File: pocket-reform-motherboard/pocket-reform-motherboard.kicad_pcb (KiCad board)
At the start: 2 copper layers, 130 x 80 mm, 20 parts, among them J1 PWR, J2 Micro_SD_Card_Det, J3 USB_C_Receptacle, J4 AudioJack4, J5 USB_C_Receptacle, J6 USBINT, J7 HDMI_D_1.4, J8 SIM, U1 reform2-som-connector, U2 MPCIE-Socket-reform-motherboa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, U3 TUSB4041I, U4 WM8960, U6 MPCIE-Socket-reform-motherboa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

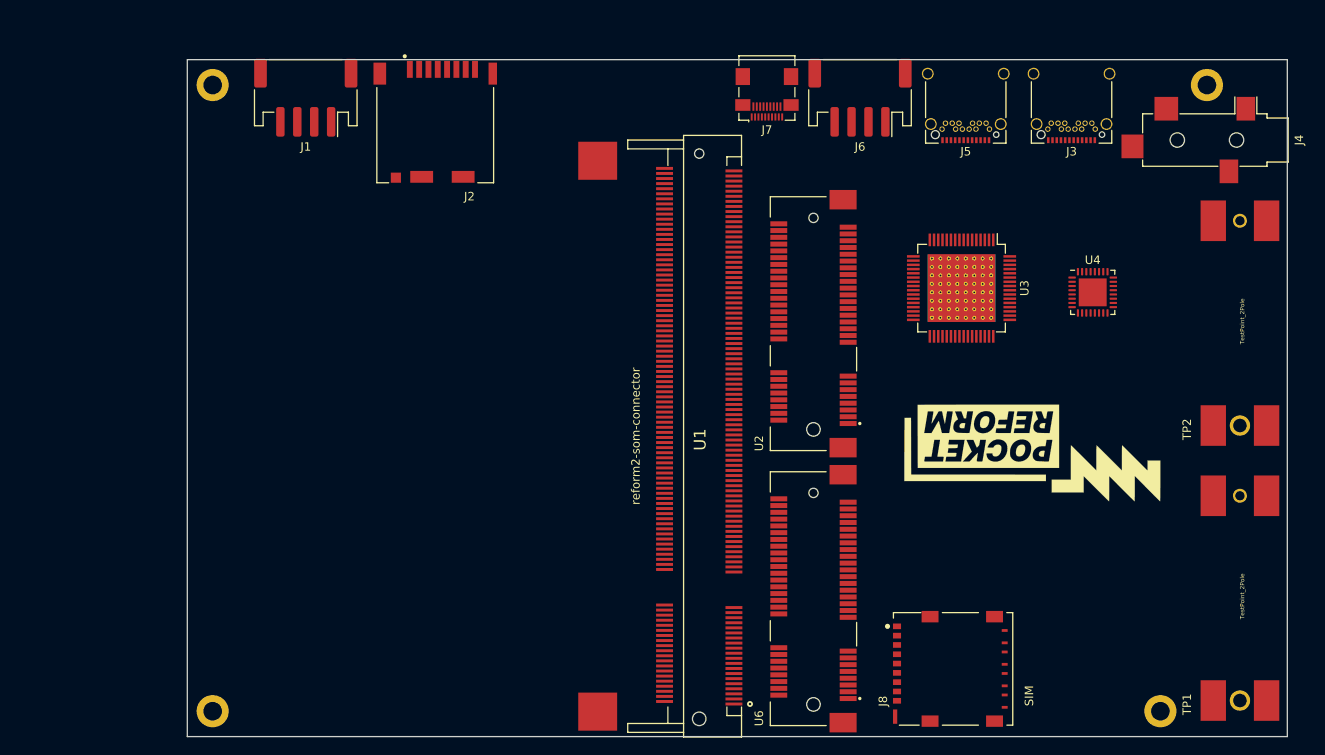
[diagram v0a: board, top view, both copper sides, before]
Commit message: motherboard D-1 first schematic and placement
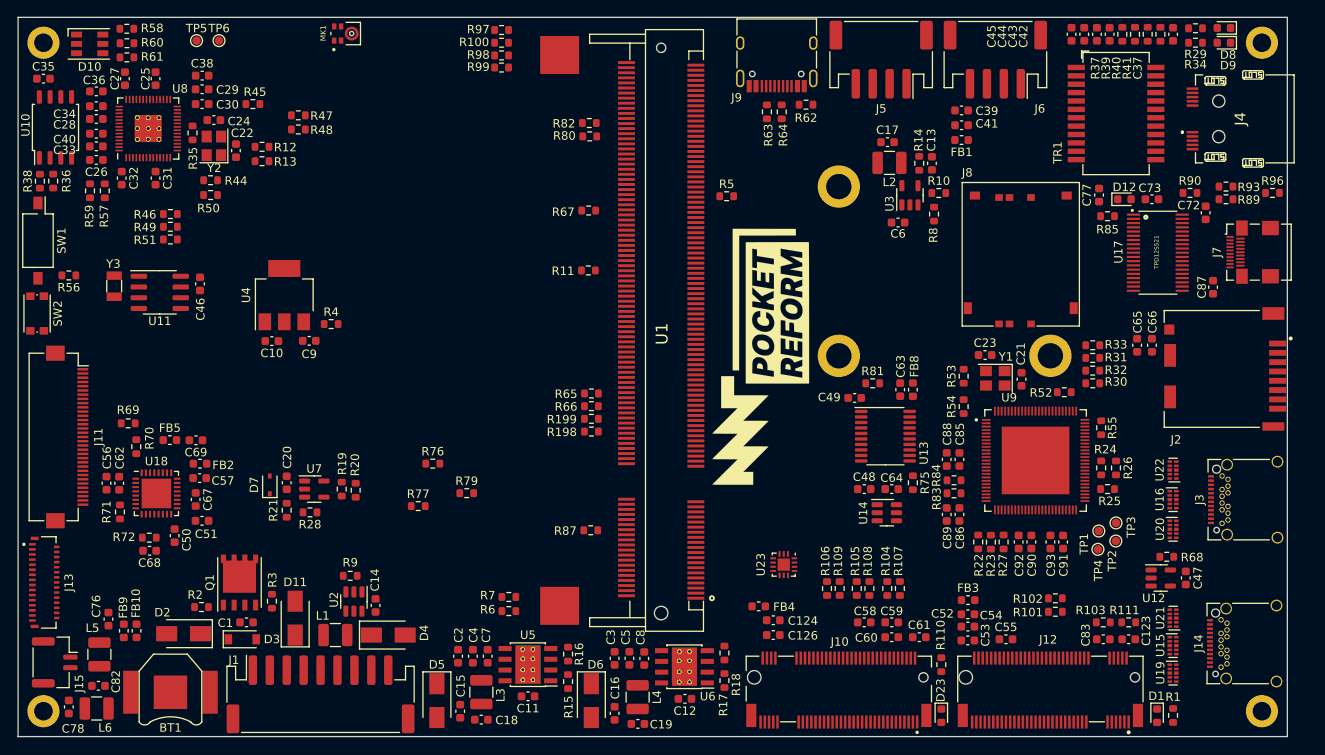
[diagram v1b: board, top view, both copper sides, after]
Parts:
- added BT1: V364, Battery:BatteryHolder_Keystone_2998_1x6.8mm, F.Cu at (77.0, 146.8)
- added C1: 0.1uF, Capacitor_SMD:C_0603_1608Metric, F.Cu at (86.0, 138.5)
- added C10: 1uF, Capacitor_SMD:C_0603_1608Metric, F.Cu at (89.0, 105.3)
- added C11: 10nF, Capacitor_SMD:C_0603_1608Metric, F.Cu at (119.3, 147.2)
- added C12: 10nF, Capacitor_SMD:C_0603_1608Metric, F.Cu at (137.8, 147.5)
- added C123: 47uF, Capacitor_SMD:C_0603_1608Metric, F.Cu at (190.2, 140.5)
- added C124: 47uF, Capacitor_SMD:C_0603_1608Metric, F.Cu at (148.2, 138.2)
- added C126: 47uF, Capacitor_SMD:C_0603_1608Metric, F.Cu at (148.2, 140.0)
- added C13: 12pF, Capacitor_SMD:C_0603_1608Metric, F.Cu at (167.0, 84.2)
- added C14: 68uF, Capacitor_SMD:C_0603_1608Metric, F.Cu at (101.2, 136.5)
- added C15: 330uF, Capacitor_SMD:C_0603_1608Metric, F.Cu at (111.2, 149.0)
- added C16: 330uF, Capacitor_SMD:C_0603_1608Metric, F.Cu at (129.5, 149.2)
- added C17: 10uF, Capacitor_SMD:C_0603_1608Metric, F.Cu at (161.8, 81.8)
- added C18: 10nF, Capacitor_SMD:C_0603_1608Metric, F.Cu at (113.8, 150.0)
- added C19: 10nF, Capacitor_SMD:C_0603_1608Metric, F.Cu at (132.2, 150.5)
- added C2: 4.7uF, Capacitor_SMD:C_0603_1608Metric, F.Cu at (111.0, 142.5)
- added C20: 1uF, Capacitor_SMD:C_0603_1608Metric, F.Cu at (90.8, 122.0)
- added C21: 18pF, Capacitor_SMD:C_0603_1608Metric, F.Cu at (177.6, 109.8)
- added C22: 27pF, Capacitor_SMD:C_0603_1608Metric, F.Cu at (84.8, 82.8)
- added C23: 18pF, Capacitor_SMD:C_0603_1608Metric, F.Cu at (173.3, 106.9)
- added C24: 27pF, Capacitor_SMD:C_0603_1608Metric, F.Cu at (82.1, 79.1)
- added C25: 0.1uF, Capacitor_SMD:C_0603_1608Metric, F.Cu at (75.2, 74.2)
- added C26: 1uF, Capacitor_SMD:C_0603_1608Metric, F.Cu at (68.2, 83.8)
- added C27: 0.1uF, Capacitor_SMD:C_0603_1608Metric, F.Cu at (71.6, 74.2)
- added C28: 0.1uF, Capacitor_SMD:C_0603_1608Metric, F.Cu at (68.2, 79.0)
- added C29: 0.1uF, Capacitor_SMD:C_0603_1608Metric, F.Cu at (80.8, 75.5)
- added C3: 4.7uF, Capacitor_SMD:C_0603_1608Metric, F.Cu at (129.5, 142.8)
- added C30: 0.1uF, Capacitor_SMD:C_0603_1608Metric, F.Cu at (80.8, 77.2)
- added C31: 0.1uF, Capacitor_SMD:C_0603_1608Metric, F.Cu at (75.2, 86.0)
- added C32: 0.1uF, Capacitor_SMD:C_0603_1608Metric, F.Cu at (71.2, 86.0)
- added C33: 0.1uF, Capacitor_SMD:C_0603_1608Metric, F.Cu at (68.2, 82.2)
- added C34: 1uF, Capacitor_SMD:C_0603_1608Metric, F.Cu at (68.2, 77.5)
- added C35: 0.1uF, Capacitor_SMD:C_0603_1608Metric, F.Cu at (62.0, 74.2)
- added C36: 1uF, Capacitor_SMD:C_0603_1608Metric, F.Cu at (68.2, 75.8)
- added C37: 1nF, Capacitor_SMD:C_0603_1608Metric, F.Cu at (195.5, 69.0)
- added C38: 0.1uF, Capacitor_SMD:C_0603_1608Metric, F.Cu at (80.8, 73.9)
- added C39: 10uF, Capacitor_SMD:C_0603_1608Metric, F.Cu at (170.5, 78.0)
- added C4: 4.7uF, Capacitor_SMD:C_0603_1608Metric, F.Cu at (112.8, 142.5)
- added C40: 0.1uF, Capacitor_SMD:C_0603_1608Metric, F.Cu at (68.2, 80.8)
- added C41: 0.1uF, Capacitor_SMD:C_0603_1608Metric, F.Cu at (170.5, 79.8)
- added C42: 0.1uF, Capacitor_SMD:C_0603_1608Metric, F.Cu at (188.0, 69.0)
- added C43: 0.1uF, Capacitor_SMD:C_0603_1608Metric, F.Cu at (186.5, 69.0)
- added C44: 0.1uF, Capacitor_SMD:C_0603_1608Metric, F.Cu at (185.0, 69.0)
- added C45: 0.1uF, Capacitor_SMD:C_0603_1608Metric, F.Cu at (183.5, 69.0)
- added C46: 0.1uF, Capacitor_SMD:C_0603_1608Metric, F.Cu at (80.5, 98.5)
- added C47: 0.1uF, Capacitor_SMD:C_0603_1608Metric, F.Cu at (197.0, 133.2)
- added C48: 0.1uF, Capacitor_SMD:C_0603_1608Metric, F.Cu at (159.0, 122.8)
- added C49: 0.1uF, Capacitor_SMD:C_0603_1608Metric, F.Cu at (157.9, 112.0)
- added C5: 4.7uF, Capacitor_SMD:C_0603_1608Metric, F.Cu at (131.2, 142.8)
- added C50: 0.1uF, Capacitor_SMD:C_0603_1608Metric, F.Cu at (77.5, 128.2)
- added C51: 10uF, Capacitor_SMD:C_0603_1608Metric, F.Cu at (80.7, 126.5)
- added C52: 10nF, Capacitor_SMD:C_0603_1608Metric, F.Cu at (171.2, 137.6)
- added C53: 0.1uF, Capacitor_SMD:C_0603_1608Metric, F.Cu at (171.2, 140.6)
- added C54: 0.1uF, Capacitor_SMD:C_0603_1608Metric, F.Cu at (171.2, 139.0)
- added C55: 0.1uF, Capacitor_SMD:C_0603_1608Metric, F.Cu at (175.8, 140.5)
- added C56: 10uF, Capacitor_SMD:C_0603_1608Metric, F.Cu at (69.5, 122.0)
- added C57: 0.1uF, Capacitor_SMD:C_0603_1608Metric, F.Cu at (80.5, 121.5)
- added C58: 10nF, Capacitor_SMD:C_0603_1608Metric, F.Cu at (159.0, 138.5)
- added C59: 0.1uF, Capacitor_SMD:C_0603_1608Metric, F.Cu at (162.2, 138.5)
- added C6: 4.7uF, Capacitor_SMD:C_0603_1608Metric, F.Cu at (163.0, 91.2)
- added C60: 0.1uF, Capacitor_SMD:C_0603_1608Metric, F.Cu at (162.2, 140.2)
- added C61: 0.1uF, Capacitor_SMD:C_0603_1608Metric, F.Cu at (165.5, 140.2)
- added C62: 0.1uF, Capacitor_SMD:C_0603_1608Metric, F.Cu at (71.0, 122.1)
- added C63: 0.1uF, Capacitor_SMD:C_0603_1608Metric, F.Cu at (163.2, 111.0)
- added C64: 0.1uF, Capacitor_SMD:C_0603_1608Metric, F.Cu at (162.2, 122.8)
- added C65: 10uF, Capacitor_SMD:C_0603_1608Metric, F.Cu at (191.2, 105.8)
- added C66: 0.1uF, Capacitor_SMD:C_0603_1608Metric, F.Cu at (193.0, 105.8)
- added C67: 10uF, Capacitor_SMD:C_0603_1608Metric, F.Cu at (80.0, 124.0)
- added C68: 0.1uF, Capacitor_SMD:C_0603_1608Metric, F.Cu at (74.5, 130.0)
- added C69: 0.1uF, Capacitor_SMD:C_0603_1608Metric, F.Cu at (80.0, 117.0)
- added C7: 10nF, Capacitor_SMD:C_0603_1608Metric, F.Cu at (114.5, 142.5)
- added C72: 0.1uF, Capacitor_SMD:C_0603_1608Metric, F.Cu at (199.3, 90.1)
- added C73: 0.1uF, Capacitor_SMD:C_0603_1608Metric, F.Cu at (193.0, 88.5)
- added C76: 0.1uF, Capacitor_SMD:C_0603_1608Metric, F.Cu at (69.7, 138.1)
- added C77: 0.1uF, Capacitor_SMD:C_0603_1608Metric, F.Cu at (186.8, 88.0)
- added C78: 0.1uF, Capacitor_SMD:C_0603_1608Metric, F.Cu at (65.0, 148.5)
- added C8: 10nF, Capacitor_SMD:C_0603_1608Metric, F.Cu at (133.0, 142.8)
- added C82: 470nF, Capacitor_SMD:C_0603_1608Metric, F.Cu at (68.5, 146.0)
- added C83: 47uF, Capacitor_SMD:C_0603_1608Metric, F.Cu at (187.2, 140.5)
- added C85: 0.1uF, Capacitor_SMD:C_0603_1608Metric, F.Cu at (170.2, 119.2)
- added C86: 0.1uF, Capacitor_SMD:C_0603_1608Metric, F.Cu at (170.2, 125.8)
- added C87: 0.1uF, Capacitor_SMD:C_0603_1608Metric, F.Cu at (200.2, 98.9)
- added C88: 0.1uF, Capacitor_SMD:C_0603_1608Metric, F.Cu at (168.8, 119.2)
- added C89: 0.1uF, Capacitor_SMD:C_0603_1608Metric, F.Cu at (168.8, 125.8)
- added C9: 1uF, Capacitor_SMD:C_0603_1608Metric, F.Cu at (93.4, 105.2)
- added C90: 0.1uF, Capacitor_SMD:C_0603_1608Metric, F.Cu at (178.8, 129.0)
- added C91: 0.1uF, Capacitor_SMD:C_0603_1608Metric, F.Cu at (182.5, 129.0)
- added C92: 0.1uF, Capacitor_SMD:C_0603_1608Metric, F.Cu at (177.2, 129.0)
- added C93: 0.1uF, Capacitor_SMD:C_0603_1608Metric, F.Cu at (181.0, 129.0)
- added D1: LED_MODEM, LED_SMD:LED_0603_1608Metric, F.Cu at (193.6, 149.5)
- added D10: 19-337/R6GHBHC-A01/2T, LED_SMD:LED_RGB_PLCC-6, F.Cu at (67.5, 70.1)
- added D11: SS54?, Diode_SMD:D_SMA, F.Cu at (91.8, 138.0)
- added D12: SD0603S040S0R2, Diode_SMD:D_0603_1608Metric, F.Cu at (189.8, 88.5)
- added D2: SMAJ36CA-E3/5A, Diode_SMD:D_SMA, F.Cu at (78.6, 139.8)
- added D23: LED_NVME, LED_SMD:LED_0603_1608Metric, F.Cu at (168.1, 149.5)
- added D3: BZT52C10, Diode_SMD:D_SOD-123, F.Cu at (85.5, 140.5)
- added D4: B540C, Diode_SMD:D_SMA, F.Cu at (102.8, 140.0)
- added D5: B540C, Diode_SMD:D_SMA, F.Cu at (108.5, 147.8)
- added D6: B540C, Diode_SMD:D_SMA, F.Cu at (126.8, 147.8)
- added D7: BZX84-C5V6,215, Diode_SMD:D_SOD-323, F.Cu at (88.8, 122.2)
- added D8: LED_Small, LED_SMD:LED_0603_1608Metric, F.Cu at (201.5, 68.2)
- added D9: LED_Small, LED_SMD:LED_0603_1608Metric, F.Cu at (201.5, 70.0)
- added FB1: 220@100MHz 1.4A, Inductor_SMD:L_0603_1608Metric, F.Cu at (170.5, 81.5)
- added FB10: 100@100MHz 3A, Inductor_SMD:L_0603_1608Metric, F.Cu at (73.0, 139.5)
- added FB2: 100@100MHz 3A, Inductor_SMD:L_0603_1608Metric, F.Cu at (80.5, 119.8)
- added FB3: 100@100MHz 3A, Inductor_SMD:L_0603_1608Metric, F.Cu at (171.3, 135.9)
- added FB4: 100@100MHz 3A, Inductor_SMD:L_0603_1608Metric, F.Cu at (146.5, 136.6)
- added FB5: 100@100MHz 3A, Inductor_SMD:L_0603_1608Metric, F.Cu at (76.9, 117.0)
- added FB8: 100@100MHz 3A, Inductor_SMD:L_0603_1608Metric, F.Cu at (164.8, 111.0)
- added FB9: 100@100MHz 3A, Inductor_SMD:L_0603_1608Metric, F.Cu at (71.5, 139.5)
- added H5: NGFF-Mount1, footprints:WA-SMSI-M2, F.Cu at (156.0, 87.0)
- added H6: NGFF-Mount1, footprints:WA-SMSI-M2, F.Cu at (156.0, 107.0)
- added H7: NGFF-Mount1, footprints:WA-SMSI-M2, F.Cu at (181.0, 107.0)
- added J10: 1-2199230-6, footprints:TE_1-2199230-6, F.Cu at (156.0, 145.0)
- added J11: Conn_01x33, Connector_FFC-FPC:Hirose_FH12-33S-0.5SH_1x33-1MP_P0.50mm_Horizontal, F.Cu at (64.8, 116.6)
- added J12: 2199230-5, footprints:TE_2199230-5, F.Cu at (181.0, 145.0)
- added J13: FH35C-31S-0.3HW(50), footprints:TE_3-2328724-1, F.Cu at (61.9, 133.8)
- added J14: USB_C_Receptacle, Connector_USB:USB_C_Receptacle_Amphenol_12401548E4-2A_CircularHoles, F.Cu at (204.9, 141.0)
- added J15: Conn_01x02, Connector_JST:JST_GH_SM02B-GHS-TB_1x02-1MP_P1.25mm_Horizontal, F.Cu at (63.3, 143.2)
- added J9: USB_C_Receptacle_USB2.0, Connector_USB:USB_C_Receptacle_HRO_TYPE-C-31-M-12, F.Cu at (148.7, 71.1)
- added L1: 47uH, Inductor_SMD:L_1210_3225Metric, F.Cu at (96.5, 140.0)
- added L2: 2.2uH, Inductor_SMD:L_1210_3225Metric, F.Cu at (162.0, 84.2)
- added L3: 15uH, Inductor_SMD:L_1210_3225Metric, F.Cu at (113.8, 146.8)
- added L4: 15uH, Inductor_SMD:L_1210_3225Metric, F.Cu at (132.2, 147.3)
- added L5: 15uH, Inductor_SMD:L_1210_3225Metric, F.Cu at (68.6, 142.3)
- added L6: 15uH, Inductor_SMD:L_1210_3225Metric, F.Cu at (68.3, 148.7)
- added MK1: MP23ABS1TR, footprints:MIC_MP23ABS1TR, F.Cu at (97.7, 68.9)
- added Q1: Si7461DP, footprints:PowerPAK_SO-8_Single_8Pads, F.Cu at (85.2, 133.8)
- added R1: 1k, Resistor_SMD:R_0603_1608Metric, F.Cu at (195.5, 149.5)
- added R10: 200k, Resistor_SMD:R_0603_1608Metric, F.Cu at (167.8, 87.8)
- added R100: 47k, Resistor_SMD:R_0603_1608Metric, F.Cu at (116.1, 70.0)
- added R101: 0, Resistor_SMD:R_0603_1608Metric, F.Cu at (181.6, 137.2)
- added R102: 0, Resistor_SMD:R_0603_1608Metric, F.Cu at (181.6, 135.7)
- added R103: 0, Resistor_SMD:R_0603_1608Metric, F.Cu at (187.2, 138.5)
- added R104: 0, Resistor_SMD:R_0603_1608Metric, F.Cu at (161.7, 134.5)
- added R105: 0, Resistor_SMD:R_0603_1608Metric, F.Cu at (158.1, 134.5)
- added R106: 0, Resistor_SMD:R_0603_1608Metric, F.Cu at (154.6, 134.5)
- added R107: 0, Resistor_SMD:R_0603_1608Metric, F.Cu at (163.2, 134.5)
- added R108: 0, Resistor_SMD:R_0603_1608Metric, F.Cu at (159.6, 134.5)
- added R109: 0, Resistor_SMD:R_0603_1608Metric, F.Cu at (156.1, 134.5)
- added R11: 0, Resistor_SMD:R_0603_1608Metric, F.Cu at (126.4, 96.9)
- added R110: 1k, Resistor_SMD:R_0603_1608Metric, F.Cu at (168.1, 143.5)
- added R111: 0, Resistor_SMD:R_0603_1608Metric, F.Cu at (190.2, 138.5)
- added R12: 0, Resistor_SMD:R_0603_1608Metric, F.Cu at (87.8, 82.3)
- added R13: 0, Resistor_SMD:R_0603_1608Metric, F.Cu at (87.8, 84.0)
- added R14: 280k, Resistor_SMD:R_0603_1608Metric, F.Cu at (165.5, 84.2)
- added R15: 10k, Resistor_SMD:R_0603_1608Metric, F.Cu at (124.0, 145.5)
- added R16: 3.16k, Resistor_SMD:R_0603_1608Metric, F.Cu at (124.0, 142.2)
- added R17: 10k, Resistor_SMD:R_0603_1608Metric, F.Cu at (142.5, 145.4)
- added R18: 5.83k, Resistor_SMD:R_0603_1608Metric, F.Cu at (142.5, 142.1)
- added R19: 1.3M, Resistor_SMD:R_0603_1608Metric, F.Cu at (97.2, 122.8)
- added R198: 49.9, Resistor_SMD:R_0603_1608Metric, F.Cu at (126.8, 116.0)
- added R199: 49.9, Resistor_SMD:R_0603_1608Metric, F.Cu at (126.8, 114.5)
- added R2: 62, Resistor_SMD:R_0603_1608Metric, F.Cu at (80.7, 136.7)
- added R20: 300k, Resistor_SMD:R_0603_1608Metric, F.Cu at (98.9, 122.9)
- added R21: 1M, Resistor_SMD:R_0603_1608Metric, F.Cu at (90.8, 125.2)
- added R22: 10k, Resistor_SMD:R_0603_1608Metric, F.Cu at (172.5, 129.0)
- added R23: DNP, Resistor_SMD:R_0603_1608Metric, F.Cu at (174.0, 129.0)
- added R24: 4.7k, Resistor_SMD:R_0603_1608Metric, F.Cu at (187.0, 120.2)
- added R25: 4.7k, Resistor_SMD:R_0603_1608Metric, F.Cu at (187.8, 122.8)
- added R26: 4.7k, Resistor_SMD:R_0603_1608Metric, F.Cu at (188.8, 120.2)
- added R27: 200k, Resistor_SMD:R_0603_1608Metric, F.Cu at (175.5, 129.0)
- added R28: 120k, Resistor_SMD:R_0603_1608Metric, F.Cu at (93.5, 125.5)
- added R29: 1k, Resistor_SMD:R_0603_1608Metric, F.Cu at (198.2, 68.3)
- added R3: 1M, Resistor_SMD:R_0603_1608Metric, F.Cu at (89.0, 136.0)
- added R30: 10k, Resistor_SMD:R_0603_1608Metric, F.Cu at (186.0, 110.2)
- added R31: 36k, Resistor_SMD:R_0603_1608Metric, F.Cu at (186.0, 107.2)
- added R32: 10k, Resistor_SMD:R_0603_1608Metric, F.Cu at (186.0, 108.8)
- added R33: 36k, Resistor_SMD:R_0603_1608Metric, F.Cu at (186.0, 105.8)
- added R34: 1k, Resistor_SMD:R_0603_1608Metric, F.Cu at (198.2, 70.0)
- added R35: 1k, Resistor_SMD:R_0603_1608Metric, F.Cu at (79.6, 80.7)
- added R36: 1k, Resistor_SMD:R_0603_1608Metric, F.Cu at (63.1, 86.3)
- added R37: 75 1%, Resistor_SMD:R_0603_1608Metric, F.Cu at (189.5, 69.0)
- added R38: 10k, Resistor_SMD:R_0603_1608Metric, F.Cu at (61.6, 86.4)
- added R39: 75 1%, Resistor_SMD:R_0603_1608Metric, F.Cu at (191.0, 69.0)
- added R4: 0, Resistor_SMD:R_0603_1608Metric, F.Cu at (96.0, 103.2)
- added R40: 75 1%, Resistor_SMD:R_0603_1608Metric, F.Cu at (192.5, 69.0)
- added R41: 75 1%, Resistor_SMD:R_0603_1608Metric, F.Cu at (194.0, 69.0)
- added R44: 0, Resistor_SMD:R_0603_1608Metric, F.Cu at (81.8, 86.2)
- added R45: 0, Resistor_SMD:R_0603_1608Metric, F.Cu at (86.8, 77.2)
- added R46: 0, Resistor_SMD:R_0603_1608Metric, F.Cu at (77.0, 90.2)
- added R47: 27.4, Resistor_SMD:R_0603_1608Metric, F.Cu at (92.1, 78.6)
- added R48: 27.4, Resistor_SMD:R_0603_1608Metric, F.Cu at (92.1, 80.2)
- added R49: 0, Resistor_SMD:R_0603_1608Metric, F.Cu at (77.0, 91.8)
- added R5: 0, Resistor_SMD:R_0603_1608Metric, F.Cu at (142.7, 88.1)
- added R50: 0, Resistor_SMD:R_0603_1608Metric, F.Cu at (81.8, 88.0)
- added R51: 0, Resistor_SMD:R_0603_1608Metric, F.Cu at (77.0, 93.2)
- added R52: 10k, Resistor_SMD:R_0603_1608Metric, F.Cu at (182.6, 111.3)
- added R53: 12k 1%, Resistor_SMD:R_0603_1608Metric, F.Cu at (170.8, 109.4)
- added R54: 10k, Resistor_SMD:R_0603_1608Metric, F.Cu at (170.8, 113.0)
- added R55: 200k, Resistor_SMD:R_0603_1608Metric, F.Cu at (187.0, 115.5)
- added R56: 10k, Resistor_SMD:R_0603_1608Metric, F.Cu at (65.0, 97.5)
- added R57: 4.7k, Resistor_SMD:R_0603_1608Metric, F.Cu at (69.2, 87.5)
- added R58: 1k, Resistor_SMD:R_0603_1608Metric, F.Cu at (71.8, 68.3)
- added R59: 4.7k, Resistor_SMD:R_0603_1608Metric, F.Cu at (67.5, 87.5)
- added R6: 100k, Resistor_SMD:R_0603_1608Metric, F.Cu at (117.0, 137.2)
- added R60: 1k, Resistor_SMD:R_0603_1608Metric, F.Cu at (71.9, 70.1)
- added R61: 1k, Resistor_SMD:R_0603_1608Metric, F.Cu at (71.9, 71.7)
- added R62: DNP, Resistor_SMD:R_0603_1608Metric, F.Cu at (152.1, 77.3)
- added R63: DNP, Resistor_SMD:R_0603_1608Metric, F.Cu at (147.5, 78.2)
- added R64: DNP, Resistor_SMD:R_0603_1608Metric, F.Cu at (149.2, 78.2)
- added R65: 49.9, Resistor_SMD:R_0603_1608Metric, F.Cu at (126.8, 111.5)
- added R66: 49.9, Resistor_SMD:R_0603_1608Metric, F.Cu at (126.8, 113.0)
- added R67: 0, Resistor_SMD:R_0603_1608Metric, F.Cu at (126.4, 89.8)
- added R68: 10k, Resistor_SMD:R_0603_1608Metric, F.Cu at (194.8, 130.8)
- added R69: 100k, Resistor_SMD:R_0603_1608Metric, F.Cu at (72.0, 115.0)
- added R7: 100k, Resistor_SMD:R_0603_1608Metric, F.Cu at (117.0, 135.5)
- added R70: 0, Resistor_SMD:R_0603_1608Metric, F.Cu at (73.0, 117.7)
- added R71: 0, Resistor_SMD:R_0603_1608Metric, F.Cu at (71.0, 125.5)
- added R72: 2k2, Resistor_SMD:R_0603_1608Metric, F.Cu at (74.5, 128.5)
- added R75: 10k, Resistor_SMD:R_0603_1608Metric, F.Cu at (164.8, 122.0)
- added R76: 33, Resistor_SMD:R_0603_1608Metric, F.Cu at (108.0, 119.7)
- added R77: 33, Resistor_SMD:R_0603_1608Metric, F.Cu at (106.3, 124.8)
- added R79: 33, Resistor_SMD:R_0603_1608Metric, F.Cu at (112.0, 123.2)
- added R8: 100k, Resistor_SMD:R_0603_1608Metric, F.Cu at (167.2, 90.2)
- added R80: 33, Resistor_SMD:R_0603_1608Metric, F.Cu at (126.6, 81.1)
- added R81: 0, Resistor_SMD:R_0603_1608Metric, F.Cu at (160.0, 110.2)
- added R82: 33, Resistor_SMD:R_0603_1608Metric, F.Cu at (126.5, 79.5)
- added R83: 0, Resistor_SMD:R_0603_1608Metric, F.Cu at (169.6, 123.2)
- added R84: 0, Resistor_SMD:R_0603_1608Metric, F.Cu at (169.6, 121.7)
- added R85: 10k, Resistor_SMD:R_0603_1608Metric, F.Cu at (187.8, 90.5)
- added R87: 100k, Resistor_SMD:R_0603_1608Metric, F.Cu at (126.7, 127.6)
- added R89: 4.7k, Resistor_SMD:R_0603_1608Metric, F.Cu at (201.8, 88.5)
- added R9: 0, Resistor_SMD:R_0603_1608Metric, F.Cu at (98.2, 133.0)
- added R90: 27k, Resistor_SMD:R_0603_1608Metric, F.Cu at (197.5, 87.8)
- added R93: 4.7k, Resistor_SMD:R_0603_1608Metric, F.Cu at (201.8, 87.0)
- added R96: 10k, Resistor_SMD:R_0603_1608Metric, F.Cu at (207.2, 87.8)
- added R97: 47k, Resistor_SMD:R_0603_1608Metric, F.Cu at (116.1, 68.5)
- added R98: 47k, Resistor_SMD:R_0603_1608Metric, F.Cu at (116.1, 71.5)
- added R99: 47k, Resistor_SMD:R_0603_1608Metric, F.Cu at (116.1, 72.9)
- added SW1: SW_DIP_x01, Button_Switch_SMD:SW_DIP_SPSTx01_Slide_Omron_A6S-110x_W8.9mm_P2.54mm, F.Cu at (61.4, 93.4)
- added SW2: RESET, Button_Switch_SMD:SW_Push_1P1T_NO_CK_KMR2, F.Cu at (61.2, 102.0)
- added TP3: PRTCTL2, TestPoint:TestPoint_Pad_D1.0mm, F.Cu at (188.8, 126.8)
- added TP4: PRTCTL4, TestPoint:TestPoint_Pad_D1.0mm, F.Cu at (186.6, 129.9)
- added TP5: TestPoint, TestPoint:TestPoint_Pad_D1.0mm, F.Cu at (80.1, 69.8)
- added TP6: TestPoint, TestPoint:TestPoint_Pad_D1.0mm, F.Cu at (82.8, 69.8)
- added TR1: TG111-MSC13LF, Transformer_SMD:Transformer_Ethernet_HALO_TG111-MSC13, F.Cu at (188.8, 78.4)
- added U10: W25Q32JVSS, Package_SO:SOIC-8_5.23x5.23mm_P1.27mm, F.Cu at (63.4, 80.0)
- added U11: PCF8523T, Package_SO:SOIC-8_3.9x4.9mm_P1.27mm, F.Cu at (75.8, 99.5)
- added U12: AP22815, Package_TO_SOT_SMD:SOT-23-5, F.Cu at (194.0, 133.3)
- added U13: TXS0108EPW, Package_SO:TSSOP-20_4.4x6.5mm_P0.65mm, F.Cu at (161.5, 116.5)
- added U14: SN74AVC1T45, Package_TO_SOT_SMD:SOT-23-6, F.Cu at (161.7, 125.5)
- added U15: TPD4E02B04DQA, Package_SON:USON-10_2.5x1.0mm_P0.5mm, F.Cu at (195.5, 141.2)
- added U16: TPD4E02B04DQA, Package_SON:USON-10_2.5x1.0mm_P0.5mm, F.Cu at (195.5, 124.0)
- added U17: TPD12S521, footprints:TSSOP50P640X120-38N, F.Cu at (193.7, 94.8)
- added U18: TLV320AIC3100, Package_DFN_QFN:VQFN-32-1EP_5x5mm_P0.5mm_EP3.5x3.5mm, F.Cu at (75.3, 123.3)
- added U19: TPD4E02B04DQA, Package_SON:USON-10_2.5x1.0mm_P0.5mm, F.Cu at (195.5, 144.5)
- added U20: TPD4E02B04DQA, Package_SON:USON-10_2.5x1.0mm_P0.5mm, F.Cu at (195.5, 127.5)
- added U21: TPD4E02B04DQA, Package_SON:USON-10_2.5x1.0mm_P0.5mm, F.Cu at (195.5, 138.0)
- added U22: TPD4E02B04DQA, Package_SON:USON-10_2.5x1.0mm_P0.5mm, F.Cu at (195.5, 120.5)
- added U23: FUSB302BMPX, Package_DFN_QFN:WQFN-14-1EP_2.5x2.5mm_P0.5mm_EP1.45x1.45mm, F.Cu at (149.5, 131.7)
- added U5: TPS5450DDAR, Package_SO:TI_SO-PowerPAD-8_ThermalVias, F.Cu at (119.2, 143.5)
- added U7: CN301, Package_TO_SOT_SMD:SOT-23-5, F.Cu at (94.0, 122.8)
- added U8: RP2040, footprints:RP2040-QFN-56, F.Cu at (74.4, 80.1)
- added U9: USB7002/KDX, footprints:QFN40P1200X1200X90-101N, F.Cu at (179.2, 119.4)
- added Y1: 25MHz, Crystal:Crystal_SMD_Abracon_ABM8G-4Pin_3.2x2.5mm, F.Cu at (174.5, 109.7)
- added Y2: 12MHz 18pF, Crystal:Crystal_SMD_3225-4Pin_3.2x2.5mm, F.Cu at (82.1, 82.2)
- added Y3: 32.768 kHz, Crystal:Crystal_SMD_3215-2Pin_3.2x1.5mm, F.Cu at (70.4, 98.8)
- J1: value PWR -> CHARGER; footprint Connector_JST:JST_PH_S4B-PH-SM4-TB_1x04-1MP_P2.00mm_Horizontal -> Connector_JST:JST_PH_S9B-PH-SM4-TB_1x09-1MP_P2.00mm_Horizontal
- J4: value AudioJack4 -> 09452812561; footprint Connector_Audio:Jack_3.5mm_CUI_SJ-3524-SMT_Horizontal -> footprints:09452812561
- J5: value USB_C_Receptacle -> SYSCTL; footprint Connector_USB:USB_C_Receptacle_Amphenol_12401548E4-2A_CircularHoles -> Connector_JST:JST_PH_S4B-PH-SM4-TB_1x04-1MP_P2.00mm_Horizontal
- J6: value USBINT -> USB_INT1
- J8: value SIM -> SIM_Card; footprint footprints:TE_2199337-5 -> footprints:MOLEX_78800-0001
- TP1: value TestPoint_2Pole -> PRTCTL1; footprint footprints:MOLEX_48099-5701 -> TestPoint:TestPoint_Pad_D1.0mm
- TP2: value TestPoint_2Pole -> PRTCTL3; footprint footprints:MOLEX_48099-5701 -> TestPoint:TestPoint_Pad_D1.0mm
- U2: value MPCIE-Socket-reform-motherboard-rescue -> MAX1837EUT33+T; footprint footprints:MOLEX_67910-5700 -> Package_TO_SOT_SMD:SOT-23-6
- U3: value TUSB4041I -> LM3674MFX-ADJ/NOPB; footprint Package_QFP:HTQFP-64-1EP_10x10mm_P0.5mm_EP8x8mm_Mask4.4x4.4mm_ThermalVias -> Package_TO_SOT_SMD:SOT-23-5
- U4: value WM8960 -> TLV1117-18; footprint Package_DFN_QFN:QFN-32-1EP_5x5mm_P0.5mm_EP3.3x3.3mm -> Package_TO_SOT_SMD:SOT-223
- U6: value MPCIE-Socket-reform-motherboard-rescue -> TPS5450DDAR; footprint footprints:MOLEX_67910-5700 -> Package_SO:TI_SO-PowerPAD-8_ThermalVias
- moved J2 97.5 mm to (201.5, 108.8), turned to 90 degrees
- moved U4 95.5 mm to (90.5, 99.8), turned to 90 degrees
- moved J1 70.5 mm to (94.8, 147.0), turned to 0 degrees
- moved J7 63.0 mm to (207.0, 94.8), turned to 90 degrees
- moved U2 62.6 mm to (98.7, 136.0), turned to -90 degrees
- moved J3 52.1 mm to (205.0, 124.0), turned to 90 degrees
- moved J8 49.6 mm to (177.5, 95.0), turned to -90 degrees
- moved GFX1 33.9 mm to (146.8, 106.8), turned to 90 degrees
- moved TP2 29.6 mm to (188.7, 128.9), turned to 0 degrees
- moved H1 20.6 mm to (62.0, 70.0)
- moved H2 20.0 mm to (62.0, 149.0)
- moved TP1 18.5 mm to (186.7, 127.7), turned to 0 degrees
- moved J6 16.6 mm to (174.5, 72.0)
- moved U6 16.5 mm to (137.8, 143.8), turned to 180 degrees
- moved U1 13.3 mm to (135.0, 104.0)
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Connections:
- net Net-(U1-Pad122) renamed IMX_UART2_RX
- net Net-(U1-Pad124) renamed IMX_UART2_TX
- net Net-(U1-Pad126) renamed IMX_UART1_RX
- net Net-(U1-Pad128) renamed IMX_UART1_TX
- net Net-(U1-Pad164) renamed BACKLIGHT_PWM
- net Net-(U1-Pad168) renamed DAC_RXFS
- net Net-(U1-Pad87) renamed IMX_RESETn
- J1 pad 1: +5V -> Net-(J1-Pad1)
- J1 pad 2: +5V -> Net-(J1-Pad1)
- J1 pad 3: GND -> VCHG
- J1 pad 4: GND -> VCHG
- J2 pad 1: SD_D2 -> Net-(J2-Pad1)
- J2 pad 2: SD_D3 -> Net-(J2-Pad2)
- J2 pad 3: SD_CMD -> Net-(J2-Pad3)
- J2 pad 5: SD_CLK -> Net-(J2-Pad5)
- J2 pad 6: Net-(J2-Pad6) -> GND
- J2 pad 7: SD_D0 -> Net-(J2-Pad7)
- J2 pad 8: SD_D1 -> Net-(J2-Pad8)
- J2 pad 9: Net-(J2-Pad9) -> SD_DET
- J3 pad A1: Net-(J3-PadA1) -> GND
- J3 pad A10: USB2_RXN -> USBH_1B_RXN
- J3 pad A11: USB2_RXP -> USBH_1B_RXP
- J3 pad A12: Net-(J3-PadA1) -> GND
- J3 pad A2: USB2_TXP -> Net-(J3-PadA2)
- J3 pad A3: USB2_TXN -> Net-(J3-PadA3)
- J3 pad A4: Net-(J3-PadA4) -> +5V
- J3 pad A6: USB12_DP -> USBH_1_DP
- J3 pad A7: USB12_DN -> USBH_1_DN
- J3 pad A8: Net-(J3-PadA8) -> unconnected-(J3-PadA8)
- J3 pad A9: Net-(J3-PadA4) -> +5V
- J3 pad B1: Net-(J3-PadA1) -> GND
- J3 pad B10: USB2_RXN -> USBH_1A_RXN
- J3 pad B11: USB2_RXP -> USBH_1A_RXP
- J3 pad B12: Net-(J3-PadA1) -> GND
- J3 pad B2: USB2_TXP -> Net-(J3-PadB2)
- J3 pad B3: USB2_TXN -> Net-(J3-PadB3)
- J3 pad B4: Net-(J3-PadA4) -> +5V
- J3 pad B6: USB12_DP -> USBH_1_DP
- J3 pad B7: USB12_DN -> USBH_1_DN
- J3 pad B8: Net-(J3-PadB8) -> unconnected-(J3-PadB8)
- J3 pad B9: Net-(J3-PadA4) -> +5V
- J3 pad S1: Net-(J3-PadS1) -> GND
- J6 pad 2: USB13_DP -> USBH_3_DN
- J6 pad 3: USB13_DN -> USBH_3_DP
- J6 pad 4: Net-(J6-Pad4) -> GND
- J7 pad 10: Net-(J7-Pad10) -> GND
- J7 pad 13: Net-(J7-Pad13) -> GND
- J7 pad 16: Net-(J7-Pad16) -> GND
- J7 pad 2: Net-(J7-Pad2) -> unconnected-(J7-Pad2)
- J7 pad 4: Net-(J7-Pad4) -> GND
- J7 pad 7: Net-(J7-Pad7) -> GND
- J7 pad SH: Net-(J7-PadSH) -> GND
- J8 pad 1: Net-(J8-Pad1) -> UIM_PWR
- J8 pad 5: Net-(J8-Pad5) -> GND
- TP1 pad 1: GND -> /PRT_CTL1
- TP2 pad 1: GND -> /PRT_CTL3
- U1 pad 10: Net-(U1-Pad10) -> unconnected-(U1-Pad10)
- U1 pad 101: Net-(U1-Pad101) -> DAC_SCL
- U1 pad 103: Net-(U1-Pad103) -> DAC_SDA
- U1 pad 104: Net-(U1-Pad104) -> GND
- U1 pad 105: Net-(U1-Pad105) -> unconnected-(U1-Pad105)
- U1 pad 107: Net-(U1-Pad107) -> unconnected-(U1-Pad107)
- U1 pad 109: Net-(U1-Pad109) -> unconnected-(U1-Pad109)
- U1 pad 11: Net-(U1-Pad11) -> ETH0_D+
- U1 pad 110: Net-(U1-Pad110) -> GND
- U1 pad 111: Net-(U1-Pad111) -> unconnected-(U1-Pad111)
- U1 pad 116: Net-(U1-Pad116) -> GND
- U1 pad 117: Net-(U1-Pad117) -> unconnected-(U1-Pad117)
- U1 pad 120: Net-(U1-Pad120) -> unconnected-(U1-Pad120)
- U1 pad 123: Net-(U1-Pad123) -> unconnected-(U1-Pad123)
- U1 pad 129: Net-(U1-Pad129) -> GND
- U1 pad 13: Net-(U1-Pad13) -> GND
- U1 pad 130: Net-(U1-Pad130) -> unconnected-(U1-Pad130)
- U1 pad 131: Net-(U1-Pad131) -> ~{USBH_RESET}
- U1 pad 132: Net-(U1-Pad132) -> unconnected-(U1-Pad132)
- U1 pad 133: Net-(U1-Pad133) -> unconnected-(U1-Pad133)
- U1 pad 134: Net-(U1-Pad134) -> unconnected-(U1-Pad134)
- U1 pad 135: Net-(U1-Pad135) -> unconnected-(U1-Pad135)
- U1 pad 136: Net-(U1-Pad136) -> unconnected-(U1-Pad136)
- U1 pad 137: Net-(U1-Pad137) -> unconnected-(U1-Pad137)
- U1 pad 138: Net-(U1-Pad138) -> unconnected-(U1-Pad138)
- U1 pad 139: Net-(U1-Pad139) -> unconnected-(U1-Pad139)
- U1 pad 140: Net-(U1-Pad140) -> unconnected-(U1-Pad140)
- U1 pad 141: Net-(U1-Pad141) -> IMX_RTC_IRQ
- U1 pad 142: Net-(U1-Pad142) -> unconnected-(U1-Pad142)
- U1 pad 143: Net-(U1-Pad143) -> unconnected-(U1-Pad143)
- U1 pad 144: Net-(U1-Pad144) -> unconnected-(U1-Pad144)
- U1 pad 145: Net-(U1-Pad145) -> IMX_WAKE
- U1 pad 146: Net-(U1-Pad146) -> unconnected-(U1-Pad146)
- U1 pad 147: Net-(U1-Pad147) -> unconnected-(U1-Pad147)
- U1 pad 148: Net-(U1-Pad148) -> unconnected-(U1-Pad148)
- U1 pad 149: Net-(U1-Pad149) -> unconnected-(U1-Pad149)
- U1 pad 15: Net-(U1-Pad15) -> ETH0_C-
- U1 pad 150: Net-(U1-Pad150) -> unconnected-(U1-Pad150)
- U1 pad 151: Net-(U1-Pad151) -> unconnected-(U1-Pad151)
- U1 pad 152: Net-(U1-Pad152) -> unconnected-(U1-Pad152)
- U1 pad 153: Net-(U1-Pad153) -> unconnected-(U1-Pad153)
- U1 pad 154: Net-(U1-Pad154) -> unconnected-(U1-Pad154)
- U1 pad 155: Net-(U1-Pad155) -> unconnected-(U1-Pad155)
- U1 pad 156: Net-(U1-Pad156) -> unconnected-(U1-Pad156)
- U1 pad 157: Net-(U1-Pad157) -> unconnected-(U1-Pad157)
- U1 pad 158: Net-(U1-Pad158) -> unconnected-(U1-Pad158)
- U1 pad 159: Net-(U1-Pad159) -> unconnected-(U1-Pad159)
- U1 pad 160: Net-(U1-Pad160) -> unconnected-(U1-Pad160)
- U1 pad 161: Net-(U1-Pad161) -> GND
- U1 pad 162: Net-(U1-Pad162) -> unconnected-(U1-Pad162)
- U1 pad 166: Net-(U1-Pad166) -> DAC_DIN
- U1 pad 167: Net-(U1-Pad167) -> GND
- U1 pad 17: Net-(U1-Pad17) -> ETH0_C+
- U1 pad 170: Net-(U1-Pad170) -> DAC_BCLK
- U1 pad 172: Net-(U1-Pad172) -> DAC_TXFS
- U1 pad 173: Net-(U1-Pad173) -> GND
- U1 pad 174: Net-(U1-Pad174) -> unconnected-(U1-Pad174)
- U1 pad 176: Net-(U1-Pad176) -> DAC_MCLK
- U1 pad 178: Net-(U1-Pad178) -> DAC_DOUT
- U1 pad 179: Net-(U1-Pad179) -> GND
- U1 pad 180: Net-(U1-Pad180) -> unconnected-(U1-Pad180)
- U1 pad 182: Net-(U1-Pad182) -> unconnected-(U1-Pad182)
- U1 pad 184: Net-(U1-Pad184) -> unconnected-(U1-Pad184)
- U1 pad 185: Net-(U1-Pad185) -> GND
- U1 pad 186: Net-(U1-Pad186) -> unconnected-(U1-Pad186)
- U1 pad 188: Net-(U1-Pad188) -> unconnected-(U1-Pad188)
- U1 pad 19: Net-(U1-Pad19) -> GND
- U1 pad 190: Net-(U1-Pad190) -> unconnected-(U1-Pad190)
- U1 pad 191: Net-(U1-Pad191) -> GND
- U1 pad 192: Net-(U1-Pad192) -> unconnected-(U1-Pad192)
- U1 pad 193: Net-(U1-Pad193) -> HDMI_SDA
- U1 pad 194: Net-(U1-Pad194) -> unconnected-(U1-Pad194)
- U1 pad 195: Net-(U1-Pad195) -> HDMI_SCL
- U1 pad 196: Net-(U1-Pad196) -> unconnected-(U1-Pad196)
- U1 pad 197: Net-(U1-Pad197) -> HDMI_CEC
- U1 pad 198: Net-(U1-Pad198) -> unconnected-(U1-Pad198)
- U1 pad 199: Net-(U1-Pad199) -> HDMI_HPD
- U1 pad 200: Net-(U1-Pad200) -> unconnected-(U1-Pad200)
- U1 pad 21: Net-(U1-Pad21) -> ETH0_B-
- U1 pad 23: Net-(U1-Pad23) -> ETH0_B+
- U1 pad 24: Net-(U1-Pad24) -> PCIE2_RESETn
- U1 pad 25: Net-(U1-Pad25) -> GND
- U1 pad 26: Net-(U1-Pad26) -> SD_DET
- U1 pad 27: Net-(U1-Pad27) -> ETH0_A-
- U1 pad 28: Net-(U1-Pad28) -> unconnected-(U1-Pad28)
- U1 pad 29: Net-(U1-Pad29) -> ETH0_A+
- U1 pad 31: Net-(U1-Pad31) -> GND
- U1 pad 33: Net-(U1-Pad33) -> unconnected-(U1-Pad33)
- U1 pad 34: Net-(U1-Pad34) -> unconnected-(U1-Pad34)
- U1 pad 35: Net-(U1-Pad35) -> unconnected-(U1-Pad35)
- U1 pad 36: Net-(U1-Pad36) -> unconnected-(U1-Pad36)
- U1 pad 37: Net-(U1-Pad37) -> PCIE1_RESETn
- U1 pad 38: Net-(U1-Pad38) -> unconnected-(U1-Pad38)
- U1 pad 39: Net-(U1-Pad39) -> unconnected-(U1-Pad39)
- U1 pad 40: Net-(U1-Pad40) -> unconnected-(U1-Pad40)
- U1 pad 41: Net-(U1-Pad41) -> GND
- U1 pad 42: Net-(U1-Pad42) -> unconnected-(U1-Pad42)
- U1 pad 43: Net-(U1-Pad43) -> unconnected-(U1-Pad43)
- U1 pad 44: Net-(U1-Pad44) -> GND
- U1 pad 45: Net-(U1-Pad45) -> unconnected-(U1-Pad45)
- U1 pad 47: Net-(U1-Pad47) -> GND
- U1 pad 49: Net-(U1-Pad49) -> unconnected-(U1-Pad49)
- U1 pad 50: Net-(U1-Pad50) -> GND
- U1 pad 51: Net-(U1-Pad51) -> unconnected-(U1-Pad51)
- U1 pad 53: Net-(U1-Pad53) -> GND
- U1 pad 55: Net-(U1-Pad55) -> unconnected-(U1-Pad55)
- U1 pad 56: Net-(U1-Pad56) -> GND
- U1 pad 57: Net-(U1-Pad57) -> unconnected-(U1-Pad57)
- U1 pad 58: Net-(U1-Pad58) -> PCIE1_CLK_P
- U1 pad 59: Net-(U1-Pad59) -> GND
- U1 pad 60: Net-(U1-Pad60) -> PCIE1_CLK_N
- U1 pad 61: Net-(U1-Pad61) -> unconnected-(U1-Pad61)
- U1 pad 62: Net-(U1-Pad62) -> GND
- U1 pad 63: Net-(U1-Pad63) -> unconnected-(U1-Pad63)
- U1 pad 64: Net-(U1-Pad64) -> PCIE2_CLK_P
- U1 pad 65: Net-(U1-Pad65) -> GND
- U1 pad 66: Net-(U1-Pad66) -> PCIE2_CLK_N
- U1 pad 67: Net-(U1-Pad67) -> unconnected-(U1-Pad67)
- U1 pad 68: Net-(U1-Pad68) -> GND
- U1 pad 69: Net-(U1-Pad69) -> unconnected-(U1-Pad69)
- U1 pad 7: Net-(U1-Pad7) -> GND
- U1 pad 70: Net-(U1-Pad70) -> PCIE2_TX_P
- U1 pad 71: Net-(U1-Pad71) -> GND
- U1 pad 72: Net-(U1-Pad72) -> PCIE2_TX_N
- U1 pad 73: Net-(U1-Pad73) -> unconnected-(U1-Pad73)
- U1 pad 74: Net-(U1-Pad74) -> GND
- U1 pad 75: Net-(U1-Pad75) -> unconnected-(U1-Pad75)
- U1 pad 76: Net-(U1-Pad76) -> PCIE2_RX_P
- U1 pad 77: Net-(U1-Pad77) -> unconnected-(U1-Pad77)
- U1 pad 78: Net-(U1-Pad78) -> PCIE2_RX_N
- U1 pad 79: Net-(U1-Pad79) -> ETH0_LED_RX
- U1 pad 8: Net-(U1-Pad8) -> unconnected-(U1-Pad8)
- U1 pad 80: Net-(U1-Pad80) -> GND
- U1 pad 81: Net-(U1-Pad81) -> unconnected-(U1-Pad81)
- U1 pad 82: Net-(U1-Pad82) -> unconnected-(U1-Pad82)
- U1 pad 83: Net-(U1-Pad83) -> ETH0_LED_LINK1
- U1 pad 84: Net-(U1-Pad84) -> unconnected-(U1-Pad84)
- U1 pad 85: Net-(U1-Pad85) -> unconnected-(U1-Pad85)
- U1 pad 86: Net-(U1-Pad86) -> unconnected-(U1-Pad86)
- U1 pad 88: Net-(U1-Pad88) -> unconnected-(U1-Pad88)
- U1 pad 89: Net-(U1-Pad89) -> LPC_SS0
- U1 pad 9: Net-(U1-Pad9) -> ETH0_D-
- U1 pad 90: Net-(U1-Pad90) -> unconnected-(U1-Pad90)
- U1 pad 91: Net-(U1-Pad91) -> LPC_MOSI
- U1 pad 92: Net-(U1-Pad92) -> unconnected-(U1-Pad92)
- U1 pad 93: Net-(U1-Pad93) -> LPC_MISO
- U1 pad 94: Net-(U1-Pad94) -> GND
- U1 pad 95: Net-(U1-Pad95) -> unconnected-(U1-Pad95)
- U1 pad 96: Net-(U1-Pad96) -> unconnected-(U1-Pad96)
- U1 pad 97: Net-(U1-Pad97) -> LPC_SCK
- U1 pad 98: Net-(U1-Pad98) -> GND
- U1 pad 99: Net-(U1-Pad99) -> unconnected-(U1-Pad99)
- U2 pad 2: Net-(U2-Pad2) -> GND
- U2 pad 3: Net-(U2-Pad3) -> VCC
- U2 pad 5: Net-(U2-Pad5) -> ~{STANDBY_SHDN}
- U2 pad 6: Net-(U2-Pad6) -> STANDBY_3V3
- U3 pad 1: Net-(U3-Pad1) -> +3V3
- U3 pad 2: +3V3 -> GND
- U3 pad 3: Net-(U3-Pad3) -> 1V2_ENABLE
- U4 pad 1: Net-(U4-Pad1) -> GND
- U4 pad 2: Net-(U4-Pad2) -> +1V8
- U4 pad 4: Net-(U4-Pad4) -> (no net)
- U6 pad 2: Net-(U6-Pad2) -> unconnected-(U6-Pad2)
- U6 pad 3: Net-(U6-Pad3) -> unconnected-(U6-Pad3)
- U6 pad 5: Net-(U6-Pad5) -> 3V3_ENABLE
- U6 pad 6: Net-(U6-Pad6) -> GND
- U6 pad 7: Net-(U6-Pad7) -> VCC
- U6 pad 9: Net-(U6-Pad9) -> GND
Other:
- board size 130 x 80 mm -> 150 x 85 mm
- net class Default removed
